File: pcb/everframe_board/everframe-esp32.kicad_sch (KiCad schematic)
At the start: 22 parts, among them J2 GSB1CA11101DSHR, SW1 SW_Push, U1 MODULE-SEEEDUINO-XIAO-ESP32S3

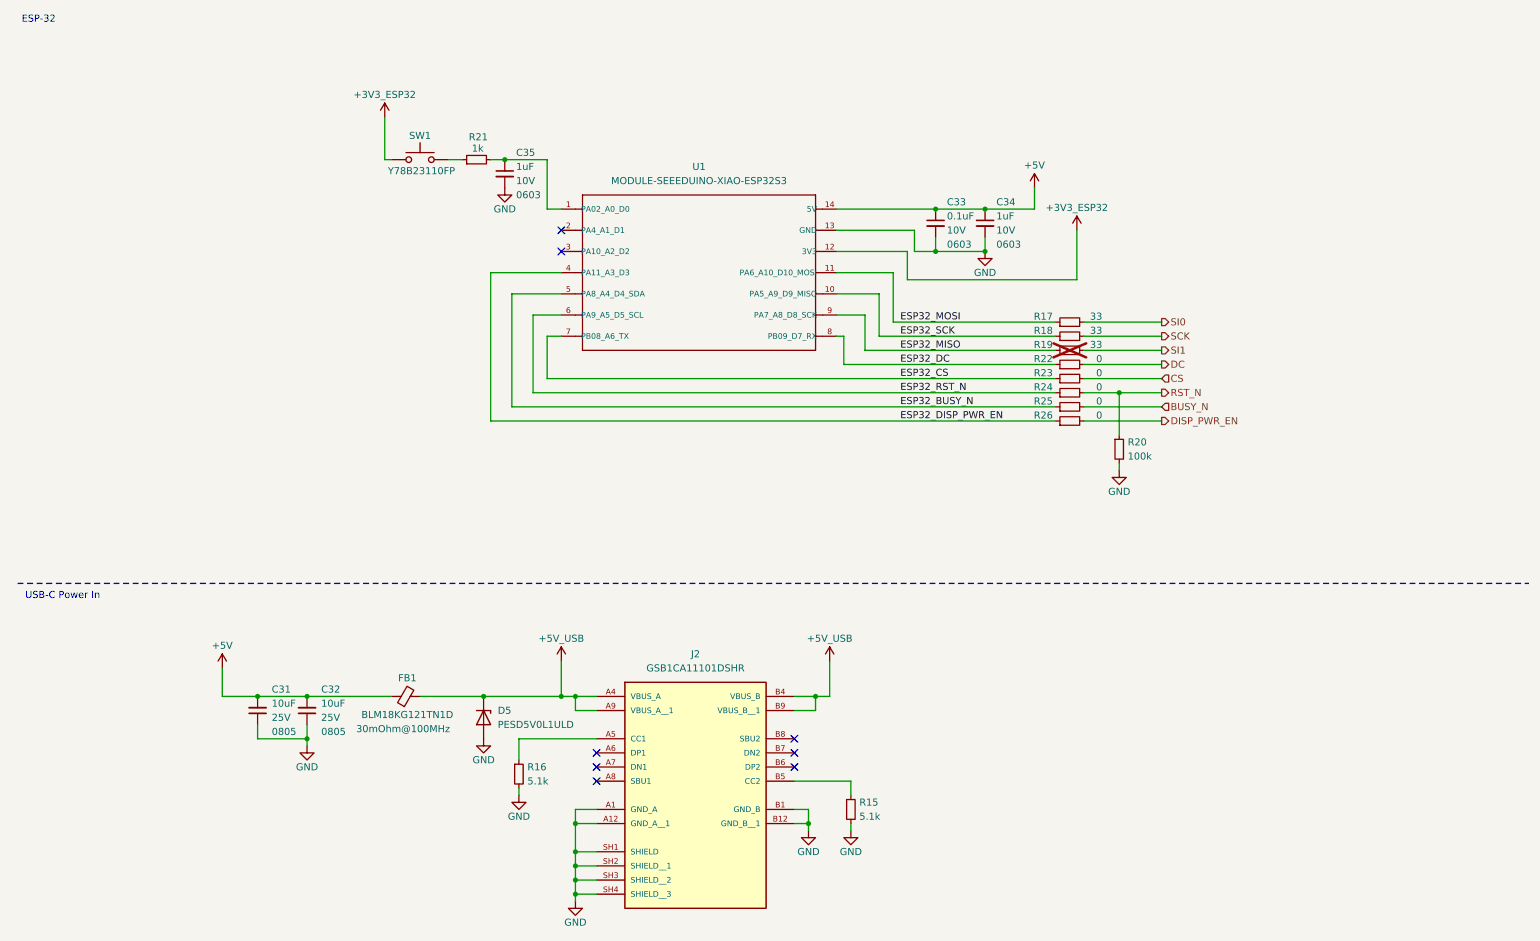
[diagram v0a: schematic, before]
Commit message: Routed board, mostly need checks
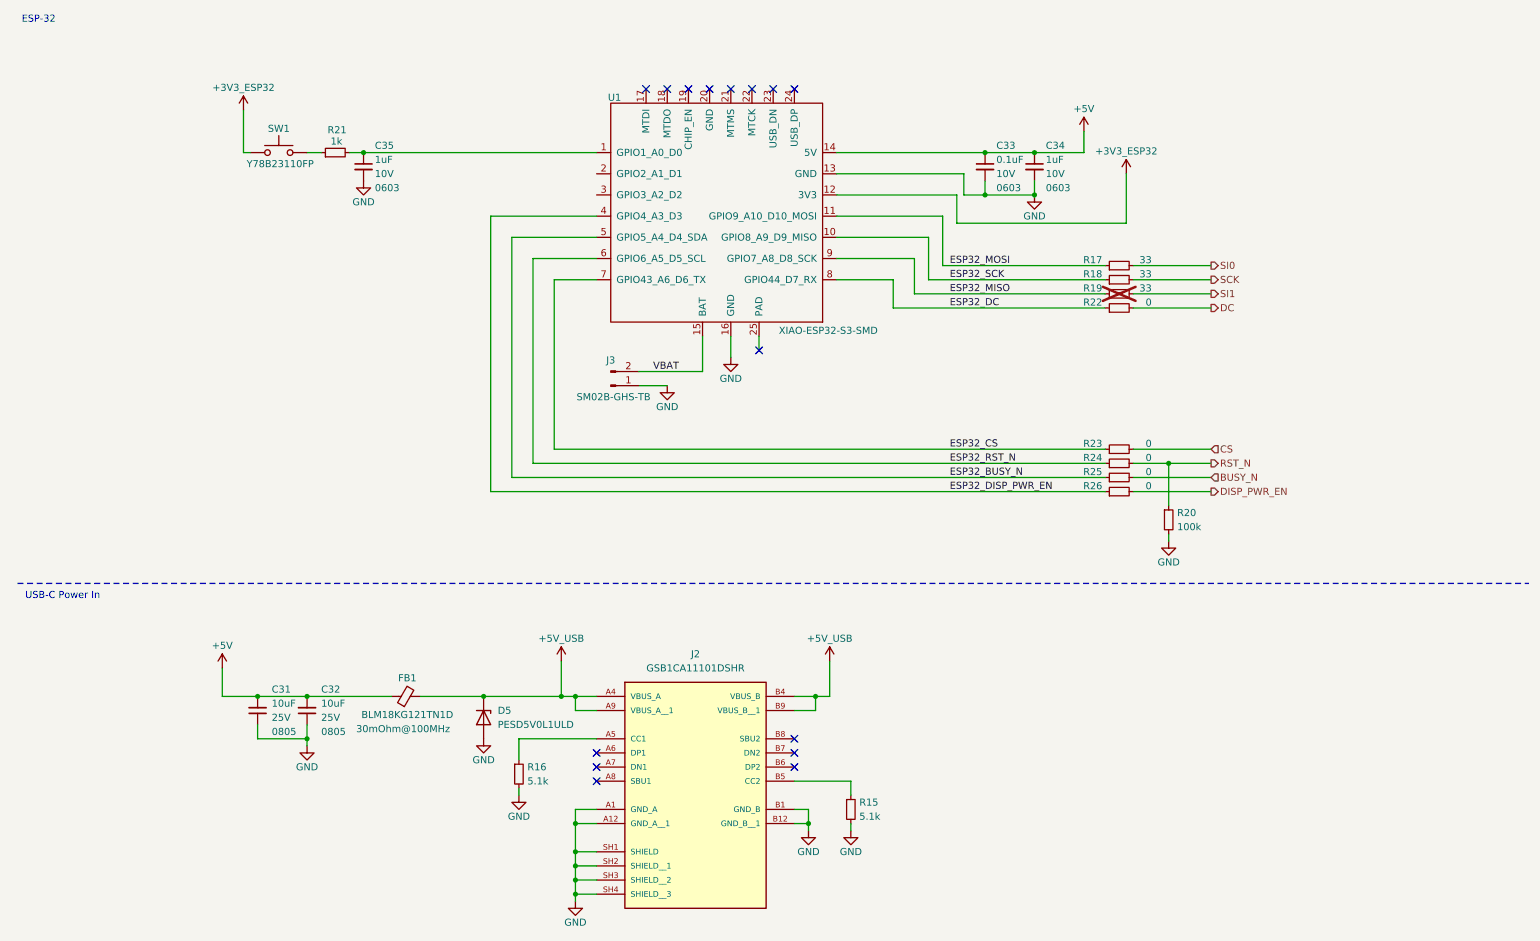
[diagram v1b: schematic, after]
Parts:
- removed U1: MODULE-SEEEDUINO-XIAO-ESP32S3, everframe_library.footprints:MOUDLE14P-SMD-2.54-21X17.8MM, symbol everframe_library:MODULE-SEEEDUINO-XIAO-ESP32S3
- added J3: SM02B-GHS-TB, Connector_JST:JST_GH_SM02B-GHS-TB_1x02-1MP_P1.25mm_Horizontal, symbol Connector:Conn_01x02_Pin
- added U1: XIAO-ESP32-S3-SMD, seed_studio:XIAO-ESP32S3-SMD, symbol xiao_seed:XIAO-ESP32-S3-SMD
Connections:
- net +3V3_ESP32: now also U1.12 (3V3)
- net +5V: now also U1.14 (5V)
- net ESP32_BUSY_N: now also U1.5 (GPIO5_A4_D4_SDA)
- net ESP32_CS: now also U1.7 (GPIO43_A6_D6_TX)
- net ESP32_DC: now also U1.8 (GPIO44_D7_RX)
- net ESP32_DISP_PWR_EN: now also U1.4 (GPIO4_A3_D3)
- net ESP32_MISO: now also U1.9 (GPIO7_A8_D8_SCK)
- net ESP32_MOSI: now also U1.11 (GPIO9_A10_D10_MOSI)
- net ESP32_RST_N: now also U1.6 (GPIO6_A5_D5_SCL)
- net ESP32_SCK: now also U1.10 (GPIO8_A9_D9_MISO)
- net GND: now also J3.1 (Pin_1), U1.13 (GND), U1.16 (GND)
- net at C35.1, R21.2: now also U1.1 (GPIO1_A0_D0)
- new net VBAT: J3.2 (Pin_2), U1.15 (BAT)
- no-connect marks 8 -> 15
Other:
- moved on the sheet: C33, C34, C35, R17, R18, R19, R20, R21, R22, R23, R24, R25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
